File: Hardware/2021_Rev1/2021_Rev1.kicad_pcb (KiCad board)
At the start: 2 copper layers, 33 parts, among them J1 USB_A, U1 TM4C129E_Launchpad, U2 OKI, U3 OKI, U4 FT230XS

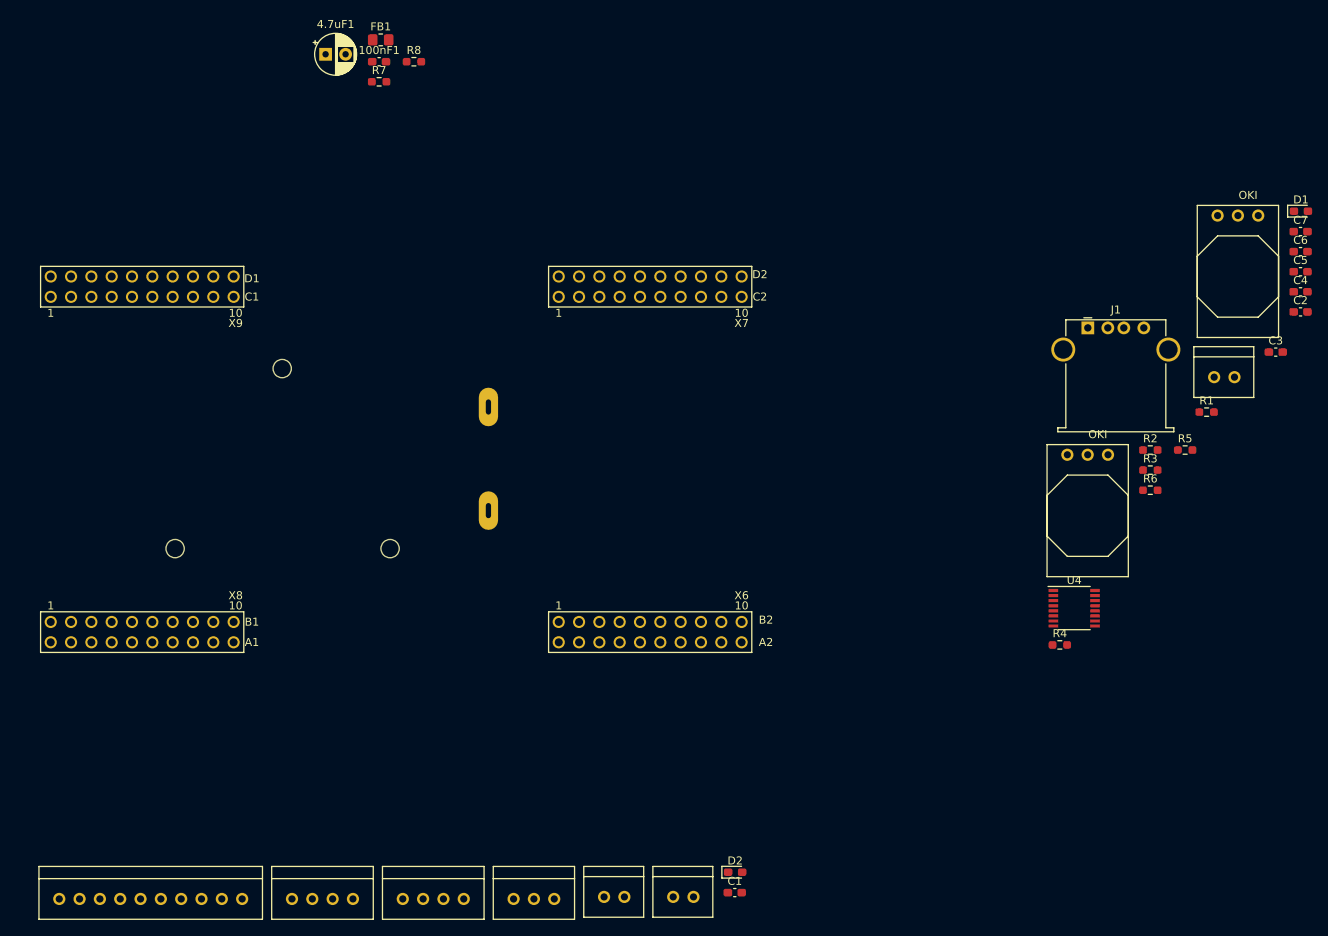
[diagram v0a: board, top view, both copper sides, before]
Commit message: Finished Layout
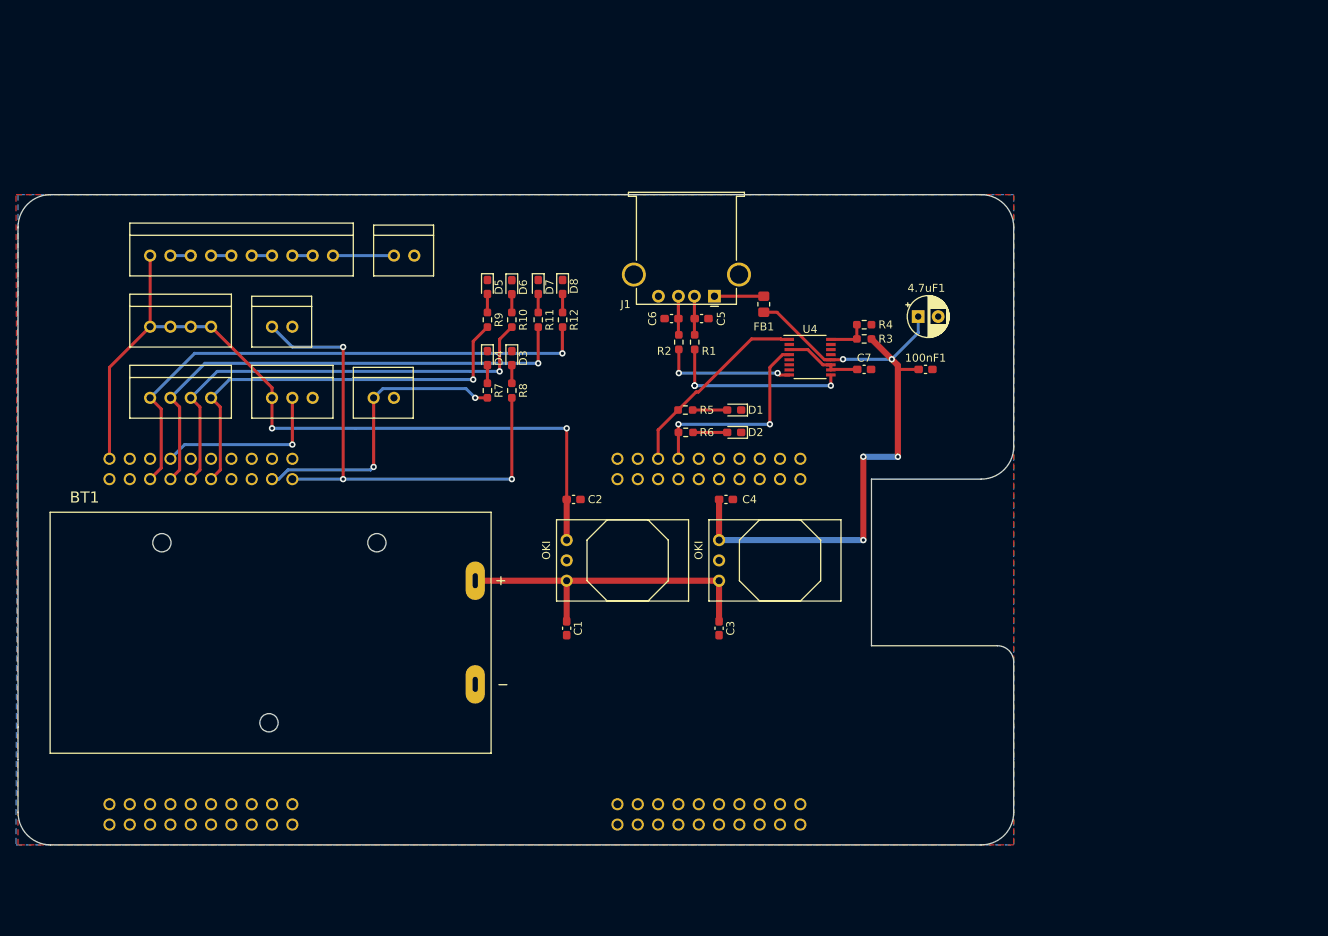
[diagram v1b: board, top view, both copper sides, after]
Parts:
- added D3: BLUE, LED_SMD:LED_0603_1608Metric_Pad1.05x0.95mm_HandSolder, F.Cu at (958.3, -224.7)
- added D4: BLUE, LED_SMD:LED_0603_1608Metric_Pad1.05x0.95mm_HandSolder, F.Cu at (955.3, -224.7)
- added D5: BLUE, LED_SMD:LED_0603_1608Metric_Pad1.05x0.95mm_HandSolder, F.Cu at (955.3, -233.6)
- added D6: BLUE, LED_SMD:LED_0603_1608Metric_Pad1.05x0.95mm_HandSolder, F.Cu at (958.3, -233.5)
- added D7: BLUE, LED_SMD:LED_0603_1608Metric_Pad1.05x0.95mm_HandSolder, F.Cu at (961.6, -233.6)
- added D8: BLUE, LED_SMD:LED_0603_1608Metric_Pad1.05x0.95mm_HandSolder, F.Cu at (964.7, -233.6)
- added R10: 330, Resistor_SMD:R_0603_1608Metric_Pad0.98x0.95mm_HandSolder, F.Cu at (958.3, -229.5)
- added R11: 330, Resistor_SMD:R_0603_1608Metric_Pad0.98x0.95mm_HandSolder, F.Cu at (961.6, -229.5)
- added R12: 330, Resistor_SMD:R_0603_1608Metric_Pad0.98x0.95mm_HandSolder, F.Cu at (964.7, -229.5)
- added R9: 330, Resistor_SMD:R_0603_1608Metric_Pad0.98x0.95mm_HandSolder, F.Cu at (955.3, -229.5)
- BT1: moved to F.Cu
- D1, D2: value PINK -> BLUE
- U1: moved to B.Cu
- moved Conn5 105.1 mm to (941.1, -219.7)
- moved C2 93.8 mm to (966.1, -207.0)
- moved Conn7 87.4 mm to (943.6, -237.5)
- moved Conn4 82.5 mm to (928.4, -228.6)
- moved Conn6 81.2 mm to (913.1, -237.5)
- moved 4.7uF1 81.0 mm to (1009.1, -229.9)
- moved C6 79.1 mm to (978.3, -229.6), turned to 180 degrees
- moved 100nF1 78.4 mm to (1010.1, -223.3)
- moved Conn3 78.2 mm to (913.1, -228.6)
- moved C3 77.7 mm to (984.2, -190.9), turned to 270 degrees
- moved U3 77.2 mm to (984.2, -196.8), turned to 90 degrees
- moved C4 76.4 mm to (985.1, -207.0)
- moved C5 75.1 mm to (982.1, -229.6)
- moved D1 75.1 mm to (986.1, -218.2), turned to 180 degrees
- moved Conn8 69.5 mm to (928.4, -219.7)
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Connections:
- 100nF1 pad 1: Net-(100nF1-Pad1) -> +5V
- 4.7uF1 pad 1: Net-(100nF1-Pad1) -> +5V
- Conn4 pad 1: Net-(Conn4-Pad1) -> ELEV_CTL
- Conn5 pad 1: Net-(Conn5-Pad1) -> AZI_CTL
- FB1 pad 1: Net-(100nF1-Pad1) -> +5V
- J1 pad 5: Net-(J1-Pad5) -> GND
- R7 pad 1: Net-(Conn5-Pad1) -> Net-(D4-Pad2)
- R8 pad 1: Net-(Conn4-Pad1) -> Net-(D3-Pad2)
- U4 pad 12: Net-(100nF1-Pad1) -> +5V
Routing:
- net +3V3: track 0.00 -> 101.8 mm, vias 0 -> 2
- net +5V: track 0.00 -> 81.8 mm, vias 0 -> 5
- net ELEV_PLUS: track 0.00 -> 68.4 mm, vias 0 -> 1
- net ELEV_CTL: track 0.00 -> 64.0 mm, vias 0 -> 3
- net ELEV_MINUS: track 0.00 -> 63.4 mm, vias 0 -> 1
- net AZI_PLUS: track 0.00 -> 57.3 mm, vias 0 -> 1
- net AZI_MINUS: track 0.00 -> 52.1 mm, vias 0 -> 1
- net +9V: track 0.00 -> 40.6 mm
- net AZI_CTL: track 0.00 -> 37.4 mm, vias 0 -> 2
- net KBoard_TX: track 0.00 -> 25.9 mm, vias 0 -> 2
- net KBoard_RX: track 0.00 -> 24.7 mm
- net Net-(R1-Pad1): track 0.00 -> 22.9 mm, vias 0 -> 3
- net LCD_TX: track 0.00 -> 21.8 mm, vias 0 -> 1
- net Net-(R2-Pad1): track 0.00 -> 16.9 mm, vias 0 -> 2
- net Net-(C7-Pad1): track 0.00 -> 9.95 mm
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- added copper zone on B.Cu, net (none)
- added copper zone on F.Cu, net GND
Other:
- board outline added: 124.5 x 81.3 mm
